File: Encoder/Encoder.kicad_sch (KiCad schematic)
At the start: 61 parts, among them J1 Conn_01x02_Male, J2 Conn_01x04_Male, J3 Conn_01x04_Male, Q1 SSM3J332R, Q12 2PB709AR, Q2 BSS138, Q3 SSM3J332R, SW1 SW_DIP_x05, SW2 SW_SPDT_White, SW3 SW_SPST, U1 AZ1084CD-3.3, U2 MAX3485, Y1 48MHz

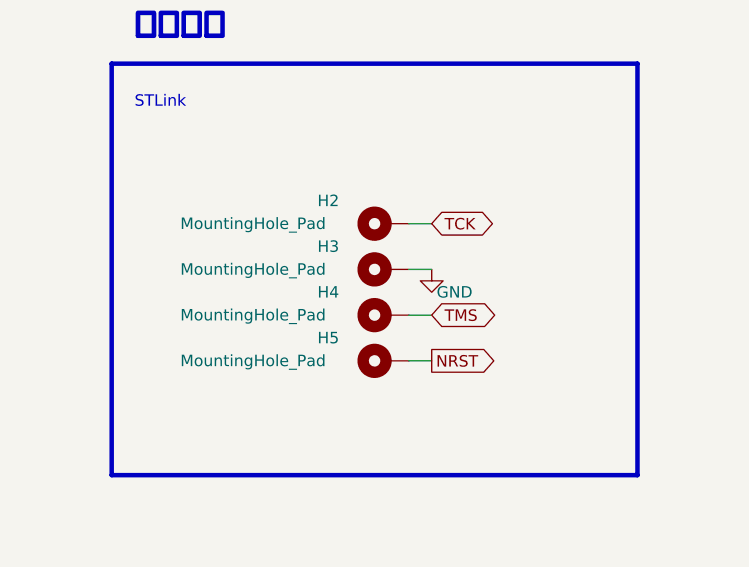
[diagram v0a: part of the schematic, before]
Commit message: 回路設計
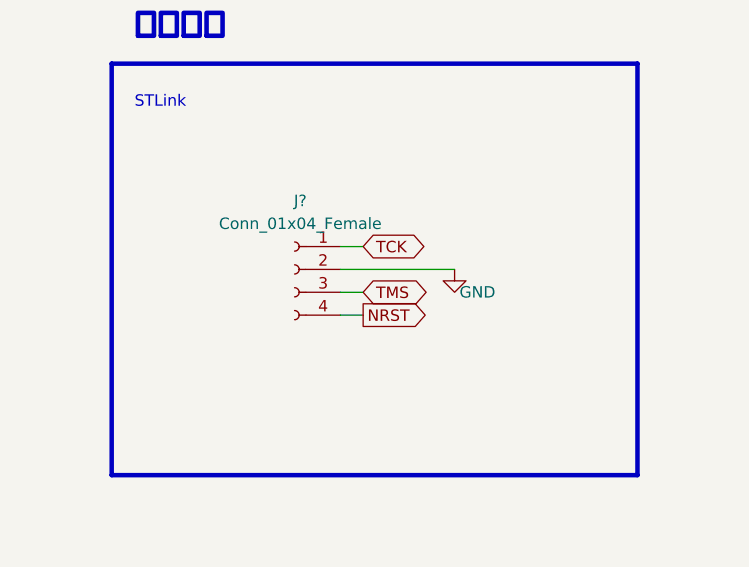
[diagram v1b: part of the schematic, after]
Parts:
- removed H2, H3, H4, H5: MountingHole_Pad, TestPoint:TestPoint_Keystone_5019_Minature, symbol Mechanical:MountingHole_Pad
- added J?: Conn_01x04_Female, Connector_PinHeader_2.54mm:PinHeader_1x04_P2.54mm_Vertical, symbol Connector:Conn_01x04_Female
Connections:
- net GND: now also J?.2 (Pin_2)
- net NRST: now also J?.4 (Pin_4)
- net TCK: now also J?.1 (Pin_1)
- net TMS: now also J?.3 (Pin_3)
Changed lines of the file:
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@@
     (stroke (width 0) (type default) (color 0 0 0 0))
   )
-  (wire (pts (xy 88.9 238.76) (xy 91.44 238.76))
+  (wire (pts (xy 81.28 236.22) (xy 83.82 236.22))
     (stroke (width 0) (type default) (color 0 0 0 0))
   )
@@
     (stroke (width 0) (type default) (color 0 0 0 0))
   )
-  (wire (pts (xy 88.9 243.84) (xy 91.44 243.84))
+  (wire (pts (xy 81.28 238.76) (xy 83.82 238.76))
     (stroke (width 0) (type default) (color 0 0 0 0))
   )
@@
     (stroke (width 0) (type default) (color 0 0 0 0))
   )
-  (wire (pts (xy 88.9 233.68) (xy 91.44 233.68))
+  (wire (pts (xy 81.28 233.68) (xy 93.98 233.68))
     (stroke (width 0) (type default) (color 0 0 0 0))
   )
@@
     (stroke (width 0) (type default) (color 0 0 0 0))
   )
-  (wire (pts (xy 88.9 228.6) (xy 91.44 228.6))
+  (wire (pts (xy 81.28 231.14) (xy 83.82 231.14))
     (stroke (width 0) (type default) (color 0 0 0 0))
   )
@@
     )
   )
-  (global_label "NRST" (shape output) (at 91.44 243.84 0) (fields_autoplaced)
-    (effects (font (size 1.27 1.27)) (justify left))
-    (property "Intersheet References" "${INTERSHEET_REFS}" (id 0) (at 50.8 66.04 0)
+  (global_label "NRST" (shape output) (at 83.82 238.76 0) (fields_autoplaced)
+    (effects (font (size 1.27 1.27)) (justify left))
+    (property "Intersheet References" "${INTERSHEET_REFS}" (id 0) (at 43.18 60.96 0)
       (effects (font (size 1.27 1.27)) hide)
     )
@@
     )
   )
-  (global_label "TCK" (shape bidirectional) (at 91.44 228.6 0) (fields_autoplaced)
-    (effects (font (size 1.27 1.27)) (justify left))
-    (property "Intersheet References" "${INTERSHEET_REFS}" (id 0) (at 50.8 58.42 0)
+  (global_label "TCK" (shape bidirectional) (at 83.82 231.14 0) (fields_autoplaced)
+    (effects (font (size 1.27 1.27)) (justify left))
+    (property "Intersheet References" "${INTERSHEET_REFS}" (id 0) (at 43.18 60.96 0)
       (effects (font (size 1.27 1.27)) hide)
     )
@@
     )
   )
-  (global_label "TMS" (shape bidirectional) (at 91.44 238.76 0) (fields_autoplaced)
-    (effects (font (size 1.27 1.27)) (justify left))
-    (property "Intersheet References" "${INTERSHEET_REFS}" (id 0) (at 50.8 63.5 0)
+  (global_label "TMS" (shape bidirectional) (at 83.82 236.22 0) (fields_autoplaced)
+    (effects (font (size 1.27 1.27)) (justify left))
+    (property "Intersheet References" "${INTERSHEET_REFS}" (id 0) (at 43.18 60.96 0)
       (effects (font (size 1.27 1.27)) hide)
     )
@@
     (pin "1")
     (pin "2")
-  )
-  (symbol (lib_id "Mechanical:MountingHole_Pad") (at 86.36 243.84 90) (mirror x) (unit 1)
-    (in_bom yes) (on_board yes)
-    (property "Reference" "H5" (id 0) (at 78.74 241.3 90)
-      (effects (font (size 1.27 1.27)) (justify right))
-    )
-    (property "Value" "MountingHole_Pad" (id 1) (at 63.5 243.84 90)
-      (effects (font (size 1.27 1.27)) (justify right))
-    )
-    (property "Footprint" "TestPoint:TestPoint_Keystone_5019_Minature" (id 2) (at 86.36 243.84 0)
-      (effects (font (size 1.27 1.27)) hide)
-    )
-    (property "Datasheet" "~" (id 3) (at 86.36 243.84 0)
-      (effects (font (size 1.27 1.27)) hide)
-    )
-    (pin "1")
   )
   (symbol (lib_id "power:+3.3V") (at 60.96 320.04 0) (unit 1)
@@
     (pin "1")
   )
-  (symbol (lib_id "Mechanical:MountingHole_Pad") (at 86.36 228.6 90) (mirror x) (unit 1)
-    (in_bom yes) (on_board yes)
-    (property "Reference" "H2" (id 0) (at 78.74 226.06 90)
-      (effects (font (size 1.27 1.27)) (justify right))
-    )
-    (property "Value" "MountingHole_Pad" (id 1) (at 63.5 228.6 90)
-      (effects (font (size 1.27 1.27)) (justify right))
-    )
-    (property "Footprint" "TestPoint:TestPoint_Keystone_5019_Minature" (id 2) (at 86.36 228.6 0)
-      (effects (font (size 1.27 1.27)) hide)
-    )
-    (property "Datasheet" "~" (id 3) (at 86.36 228.6 0)
-      (effects (font (size 1.27 1.27)) hide)
-    )
-    (pin "1")
-  )
   (symbol (lib_id "power:GND") (at 60.96 144.78 0) (unit 1)
     (in_bom yes) (on_board yes) (fields_autoplaced)
@@
     (pin "1")
     (pin "2")
-  )
-  (symbol (lib_id "Mechanical:MountingHole_Pad") (at 86.36 233.68 90) (mirror x) (unit 1)
-    (in_bom yes) (on_board yes)
-    (property "Reference" "H3" (id 0) (at 78.74 231.14 90)
-      (effects (font (size 1.27 1.27)) (justify right))
-    )
-    (property "Value" "MountingHole_Pad" (id 1) (at 63.5 233.68 90)
-      (effects (font (size 1.27 1.27)) (justify right))
-    )
-    (property "Footprint" "TestPoint:TestPoint_Keystone_5019_Minature" (id 2) (at 86.36 233.68 0)
-      (effects (font (size 1.27 1.27)) hide)
-    )
-    (property "Datasheet" "~" (id 3) (at 86.36 233.68 0)
-      (effects (font (size 1.27 1.27)) hide)
-    )
-    (pin "1")
   )
   (symbol (lib_id "Connector:TestPoint") (at 152.4 152.4 180) (unit 1)
@@
     (pin "2")
   )
-  (symbol (lib_id "power:GND") (at 91.44 233.68 0) (unit 1)
-    (in_bom yes) (on_board yes)
-    (property "Reference" "#PWR0109" (id 0) (at 91.44 240.03 0)
-      (effects (font (size 1.27 1.27)) hide)
-    )
-    (property "Value" "GND" (id 1) (at 93.98 236.22 0))
-    (property "Footprint" "" (id 2) (at 91.44 233.68 0)
-      (effects (font (size 1.27 1.27)) hide)
-    )
-    (property "Datasheet" "" (id 3) (at 91.44 233.68 0)
+  (symbol (lib_id "power:GND") (at 93.98 233.68 0) (unit 1)
+    (in_bom yes) (on_board yes)
+    (property "Reference" "#PWR0109" (id 0) (at 93.98 240.03 0)
+      (effects (font (size 1.27 1.27)) hide)
+    )
+    (property "Value" "GND" (id 1) (at 96.52 236.22 0))
+    (property "Footprint" "" (id 2) (at 93.98 233.68 0)
+      (effects (font (size 1.27 1.27)) hide)
+    )
+    (property "Datasheet" "" (id 3) (at 93.98 233.68 0)
       (effects (font (size 1.27 1.27)) hide)
     )
@@
     (pin "1")
   )
-  (symbol (lib_id "Mechanical:MountingHole_Pad") (at 86.36 238.76 90) (mirror x) (unit 1)
-    (in_bom yes) (on_board yes)
-    (property "Reference" "H4" (id 0) (at 78.74 236.22 90)
-      (effects (font (size 1.27 1.27)) (justify right))
-    )
-    (property "Value" "MountingHole_Pad" (id 1) (at 63.5 238.76 90)
-      (effects (font (size 1.27 1.27)) (justify right))
-    )
-    (property "Footprint" "TestPoint:TestPoint_Keystone_5019_Minature" (id 2) (at 86.36 238.76 0)
-      (effects (font (size 1.27 1.27)) hide)
-    )
-    (property "Datasheet" "~" (id 3) (at 86.36 238.76 0)
-      (effects (font (size 1.27 1.27)) hide)
-    )
-    (pin "1")
-  )
   (symbol (lib_id "power:VDD") (at 152.4 149.86 0) (unit 1)
     (in_bom yes) (on_board yes) (fields_autoplaced)
@@
     )
     (pin "1")
+  )
+  (symbol (lib_id "Connector:Conn_01x04_Female") (at 76.2 233.68 0) (mirror y) (unit 1)
+    (in_bom yes) (on_board yes) (fields_autoplaced)
+    (property "Reference" "J?" (id 0) (at 76.835 226.06 0))
+    (property "Value" "Conn_01x04_Female" (id 1) (at 76.835 228.6 0))
+    (property "Footprint" "Connector_PinHeader_2.54mm:PinHeader_1x04_P2.54mm_Vertical" (id 2) (at 76.2 233.68 0)
+      (effects (font (size 1.27 1.27)) hide)
+    )
+    (property "Datasheet" "~" (id 3) (at 76.2 233.68 0)
+      (effects (font (size 1.27 1.27)) hide)
+    )
+    (pin "1")
+    (pin "2")
+    (pin "3")
+    (pin "4")
   )
   (symbol (lib_id "Connector:TestPoint") (at 172.72 152.4 180) (unit 1)
@@
       (reference "D?") (unit 1) (value "SBR1A40SA") (footprint "Diode_SMD:D_SMA_Handsoldering")
     )
-    (path "/51b101dc-3fd8-439d-ba1a-45dee2ee1e7b"
-      (reference "H2") (unit 1) (value "MountingHole_Pad") (footprint "TestPoint:TestPoint_Keystone_5019_Minature")
-    )
-    (path "/5c96fa03-528c-4014-a8f5-77eb363f51fb"
-      (reference "H3") (unit 1) (value "MountingHole_Pad") (footprint "TestPoint:TestPoint_Keystone_5019_Minature")
-    )
-    (path "/d87199d4-5a00-485e-b489-b46c49d12f4d"
-      (reference "H4") (unit 1) (value "MountingHole_Pad") (footprint "TestPoint:TestPoint_Keystone_5019_Minature")
-    )
-    (path "/0a0b4be0-d712-4820-ad45-b5f3164cf350"
-      (reference "H5") (unit 1) (value "MountingHole_Pad") (footprint "TestPoint:TestPoint_Keystone_5019_Minature")
-    )
     (path "/748f3f23-7352-40c9-8bc7-ffe8531b9c38"
       (reference "H8") (unit 1) (value "MountingHole_Pad") (footprint "TestPoint:TestPoint_Pad_1.5x1.5mm")
@@
       (reference "J3") (unit 1) (value "Conn_01x04_Male") (footprint "Connector_Molex:Molex_SPOX_5268-04A_1x04_P2.50mm_Horizontal")
     )
+    (path "/e00540e1-46e4-4278-8f7c-20405075d788"
+      (reference "J?") (unit 1) (value "Conn_01x04_Female") (footprint "Connector_PinHeader_2.54mm:PinHeader_1x04_P2.54mm_Vertical")
+    )
     (path "/837550e3-e9e9-40db-91e8-a23399732e65"
